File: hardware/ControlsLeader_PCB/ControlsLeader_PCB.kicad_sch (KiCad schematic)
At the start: 11 parts, among them J1 CarCANConnector_Out, J11 Nanofit_2Rows-19Pins, J2 PeripheralCAN_out, J3 CarCANConnector_In, J4 PeripheralCAN_in, J7 Dash_LSOM_PWR, U1 LeaderSOM

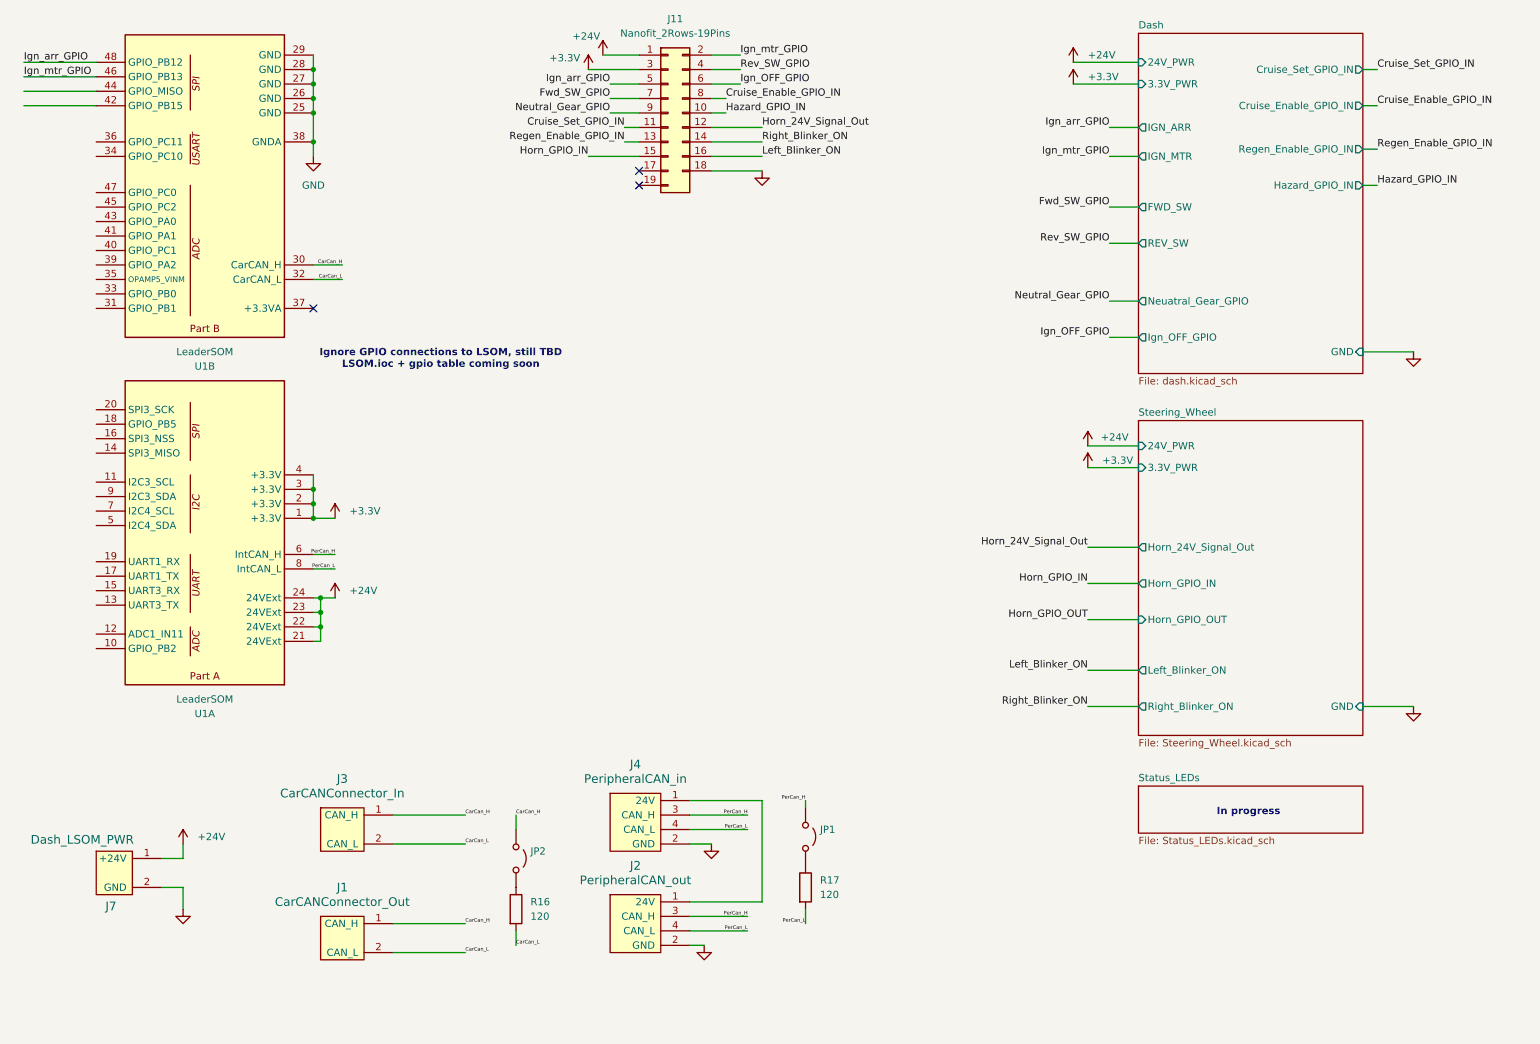
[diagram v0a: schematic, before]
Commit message: Schematic Backup
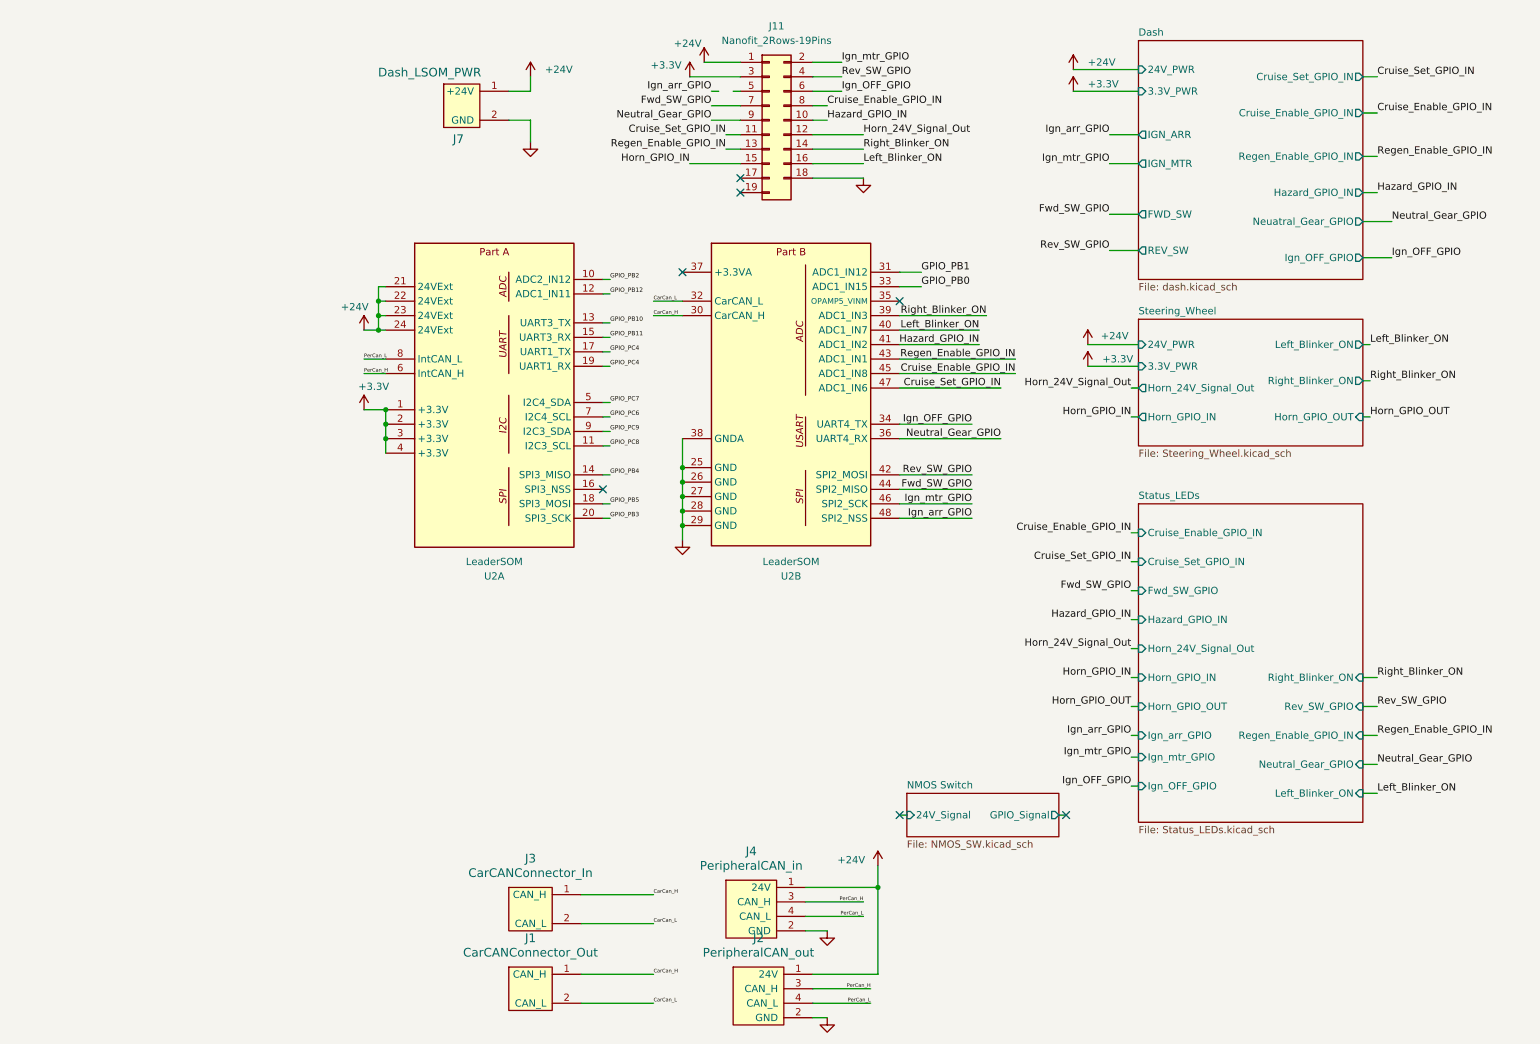
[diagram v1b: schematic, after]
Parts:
- removed JP1, JP2: Jumper_2_Open, symbol Jumper:Jumper_2_Open
- removed R16, R17: 120, symbol Device:R
- removed U1: LeaderSOM, UTSVT_Special:LeaderSOM, symbol utsvt_connectors:LeaderSOMConnector
- added U2: LeaderSOM, UTSVT_Special:LeaderSOM, symbol utsvt_connectors:LeaderSOMConnector
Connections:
- net +24V: now also J2.1 (24V), J4.1 (24V), U2.21 (24VExt), U2.22 (24VExt), U2.23 (24VExt), U2.24 (24VExt)
- net +3.3V: now also U2.1 (+3.3V), U2.2 (+3.3V), U2.3 (+3.3V), U2.4 (+3.3V)
- net CarCan_H: now also U2.30 (CarCAN_H)
- net CarCan_L: now also U2.32 (CarCAN_L)
- net Cruise_Enable_GPIO_IN: now also U2.45 (ADC1_IN8)
- net Cruise_Set_GPIO_IN: now also U2.47 (ADC1_IN6)
- net Fwd_SW_GPIO: now also U2.44 (SPI2_MISO)
- net GND: now also U2.25 (GND), U2.26 (GND), U2.27 (GND), U2.28 (GND), U2.29 (GND), U2.38 (GNDA)
- net Hazard_GPIO_IN: now also U2.41 (ADC1_IN2)
- net Ign_OFF_GPIO: now also U2.34 (UART4_TX)
- net Ign_arr_GPIO: now also U2.48 (SPI2_NSS); no longer J11.5 (Pin_5)
- net Ign_mtr_GPIO: now also U2.46 (SPI2_SCK)
- net Left_Blinker_ON: now also U2.40 (ADC1_IN7)
- net Neutral_Gear_GPIO: now also U2.36 (UART4_RX)
- net PerCan_H: now also U2.6 (IntCAN_H)
- net PerCan_L: now also U2.8 (IntCAN_L)
- net Regen_Enable_GPIO_IN: now also U2.43 (ADC1_IN1)
- net Rev_SW_GPIO: now also U2.42 (SPI2_MOSI)
- net Right_Blinker_ON: now also U2.39 (ADC1_IN3)
- new net GPIO_PB0: U2.33 (ADC1_IN15)
- new net GPIO_PB1: U2.31 (ADC1_IN12)
- new net GPIO_PB10: U2.13 (UART3_TX)
- new net GPIO_PB11: U2.15 (UART3_RX)
- new net GPIO_PB12: U2.12 (ADC1_IN11)
- new net GPIO_PB2: U2.10 (ADC2_IN12)
- new net GPIO_PB3: U2.20 (SPI3_SCK)
- new net GPIO_PB4: U2.14 (SPI3_MISO)
- new net GPIO_PB5: U2.18 (SPI3_MOSI)
- new net GPIO_PC4: U2.17 (UART1_TX), U2.19 (UART1_RX)
- new net GPIO_PC6: U2.7 (I2C4_SCL)
- new net GPIO_PC7: U2.5 (I2C4_SDA)
- new net GPIO_PC8: U2.11 (I2C3_SCL)
- new net GPIO_PC9: U2.9 (I2C3_SDA)
- no-connect marks 3 -> 7
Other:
- added sheet NMOS Switch (NMOS_SW.kicad_sch)
- sheet Dash ports: added none; removed GND
- sheet Status_LEDs ports: added Cruise_Enable_GPIO_IN, Cruise_Set_GPIO_IN, Fwd_SW_GPIO, Hazard_GPIO_IN, Horn_24V_Signal_Out, Horn_GPIO_IN, Horn_GPIO_OUT, Ign_OFF_GPIO, Ign_arr_GPIO, Ign_mtr_GPIO, Left_Blinker_ON, Neutral_Gear_GPIO, Regen_Enable_GPIO_IN, Rev_SW_GPIO, Right_Blinker_ON; removed none
- sheet Steering_Wheel ports: added none; removed GND
- note removed: "Ignore GPIO connections to LSOM, still TBD LSOM.ioc + gpio table coming soon"
- note removed: "In progress"
- moved on the sheet: J1, J11, J2, J3, J4, J7
